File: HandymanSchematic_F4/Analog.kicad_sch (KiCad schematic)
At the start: 36 parts, among them Q1 BC847, U2 TL074, U6 TL072

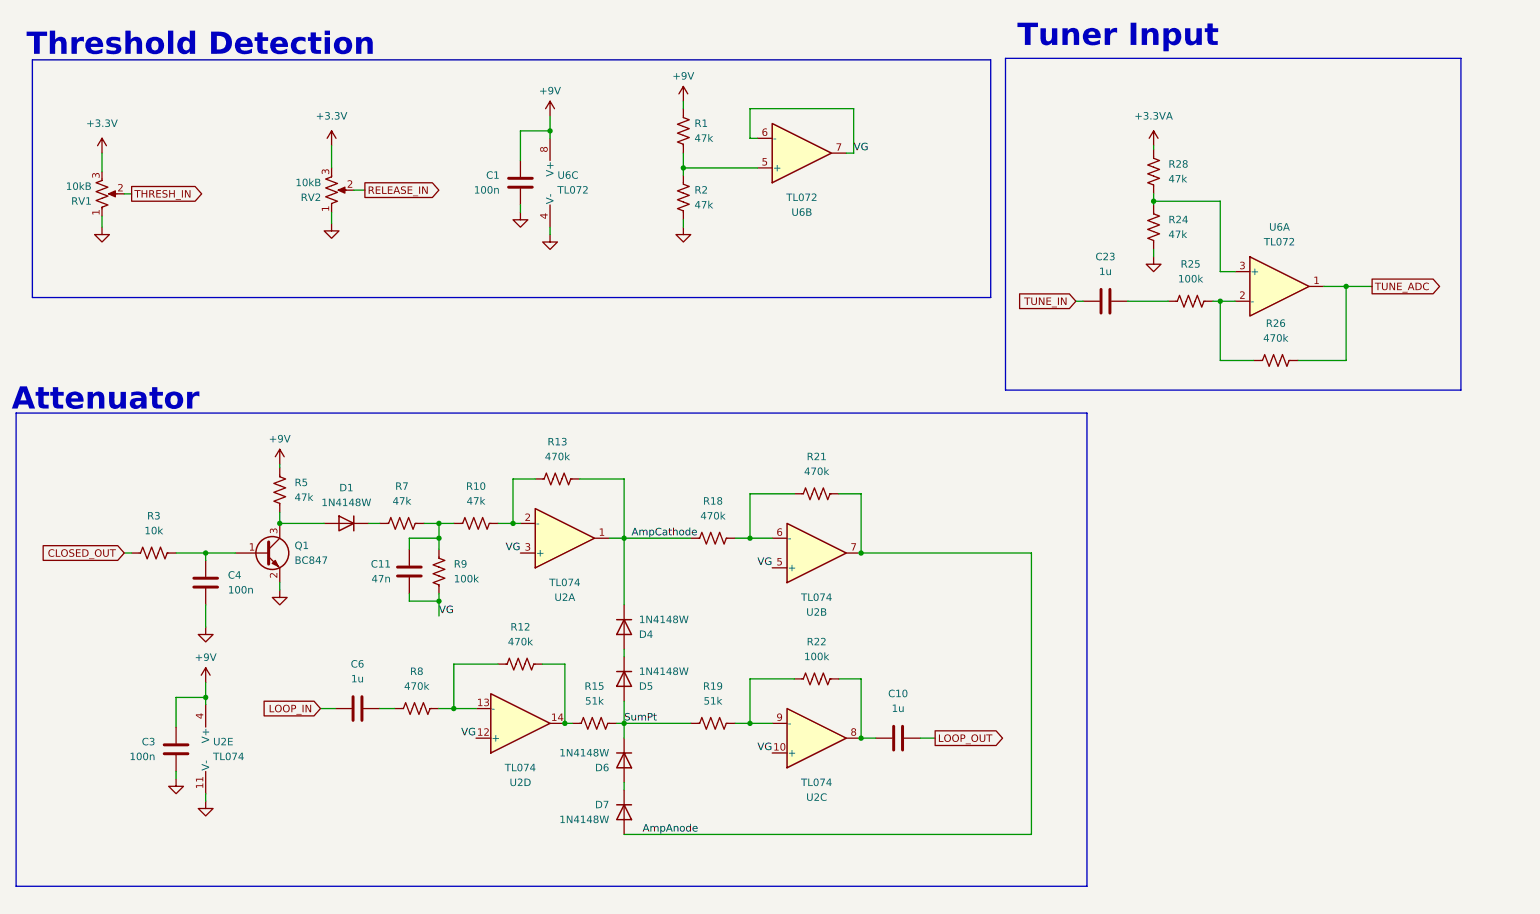
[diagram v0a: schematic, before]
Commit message: noise schematic tweaks
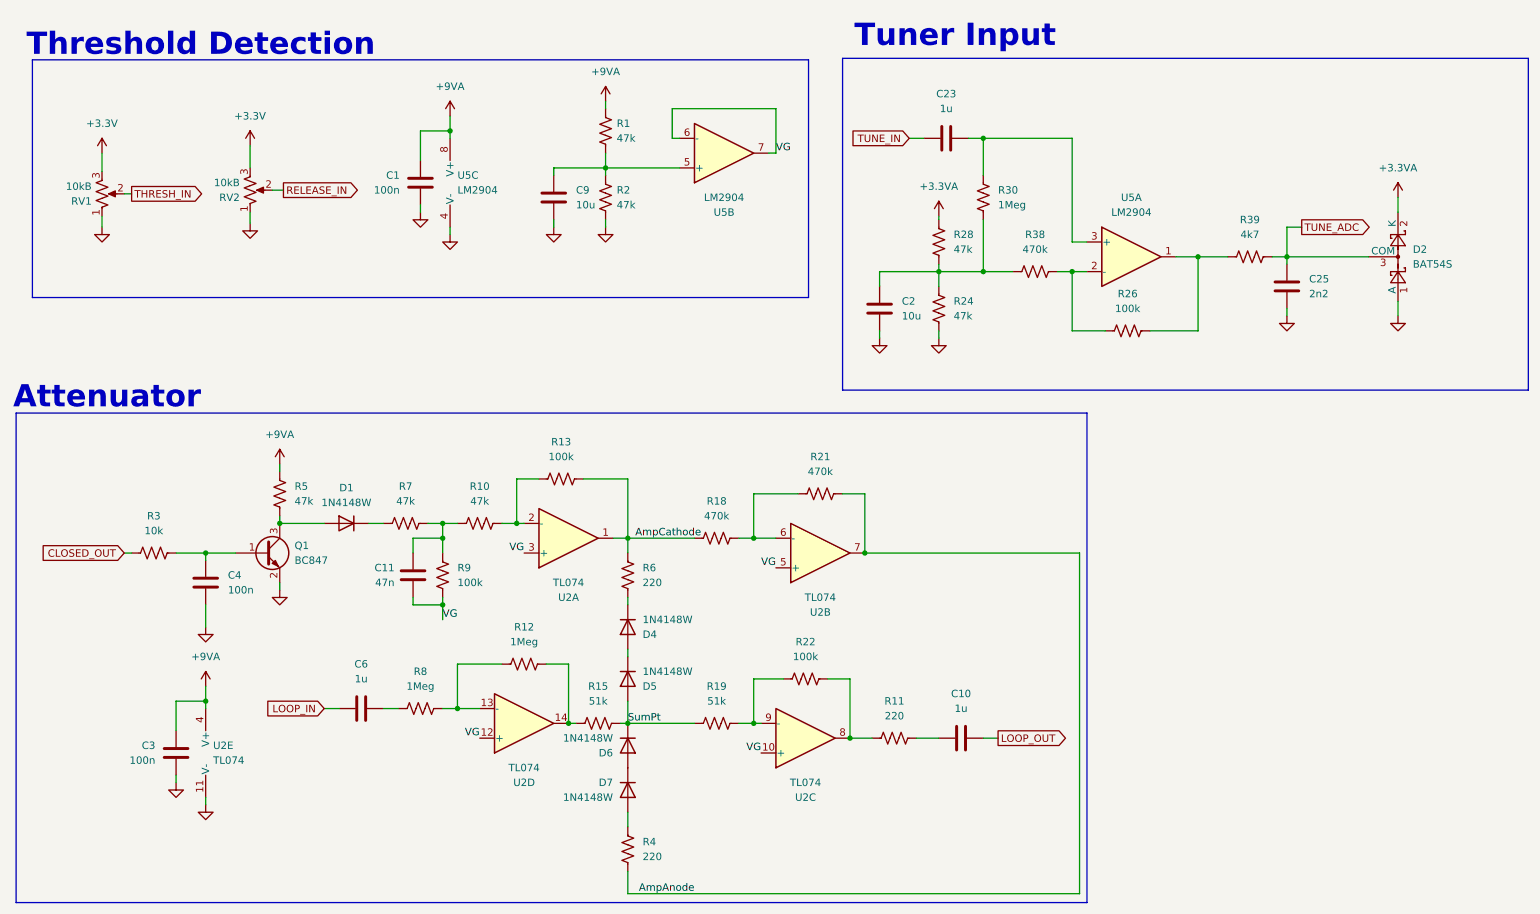
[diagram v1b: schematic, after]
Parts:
- removed R25: 100k, Resistor_SMD:R_0805_2012Metric, symbol Device:R_US
- removed U6: TL072, Package_SO:SOIC-8_3.9x4.9mm_P1.27mm, symbol Amplifier_Operational:TL072
- added C2, C9: 10u, Capacitor_SMD:C_0805_2012Metric, symbol Device:C
- added C25: 2n2, Capacitor_SMD:C_0805_2012Metric, symbol Device:C
- added D2: BAT54S, Package_TO_SOT_SMD:SOT-23, symbol Diode:BAT54S
- added R11, R4, R6: 220, Resistor_SMD:R_0805_2012Metric, symbol Device:R_US
- added R30: 1Meg, Resistor_SMD:R_0805_2012Metric, symbol Device:R_US
- added R38: 470k, Resistor_SMD:R_0805_2012Metric, symbol Device:R_US
- added R39: 4k7, Resistor_SMD:R_0805_2012Metric, symbol Device:R_US
- added U5: LM2904, Package_SO:SOIC-8_3.9x4.9mm_P1.27mm, symbol Amplifier_Operational:LM2904
- R12, R8: value 470k -> 1Meg
- R13, R26: value 470k -> 100k
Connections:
- net +3.3VA: now also D2.2 (K)
- net AmpAnode: now also R4.2; no longer D7.2 (A)
- net AmpCathode: now also R6.1; no longer D4.1 (K)
- net GND: now also C2.2, C25.2, C9.2, D2.1 (A), U5.4 (V-)
- net TUNE_ADC: now also C25.1, D2.3 (COM), R39.2; no longer R26.2
- net VG: now also U5.6 (-), U5.7
- net at R26.1: now also R38.2, U5.2 (-)
- net at R24.1, R28.2: now also C2.1, R30.2, R38.1
- net at R1.2, R2.1: now also C9.1, U5.5 (+)
- net at C23.2: now also R30.1, U5.3 (+)
- net at R22.2, U2.8: now also R11.1; no longer C10.1
- net +9V renamed +9VA
- net +9VA: now also U5.8 (V+)
- new net: D4.1 (K), R6.2
- new net: D7.2 (A), R4.1
- new net: C10.1, R11.2
- new net: R26.2, R39.1, U5.1
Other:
- moved on the sheet: C1, C10, C11, C23, C3, C6, D4, D5, D6, D7, R1, R10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
